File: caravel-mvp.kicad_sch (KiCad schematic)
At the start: 47 parts, among them J2 Conn_01x02, J3 Conn_02x04_Odd_Even, J4 Conn_01x06, J6 Conn_02x18_Odd_Even, J6 USB_C_Receptacle_USB2.0, J9 613012243121, SW3 B3U-1000P, U1 Caravel_QFN, U1 W25Q32JVSS, X1 10MHz

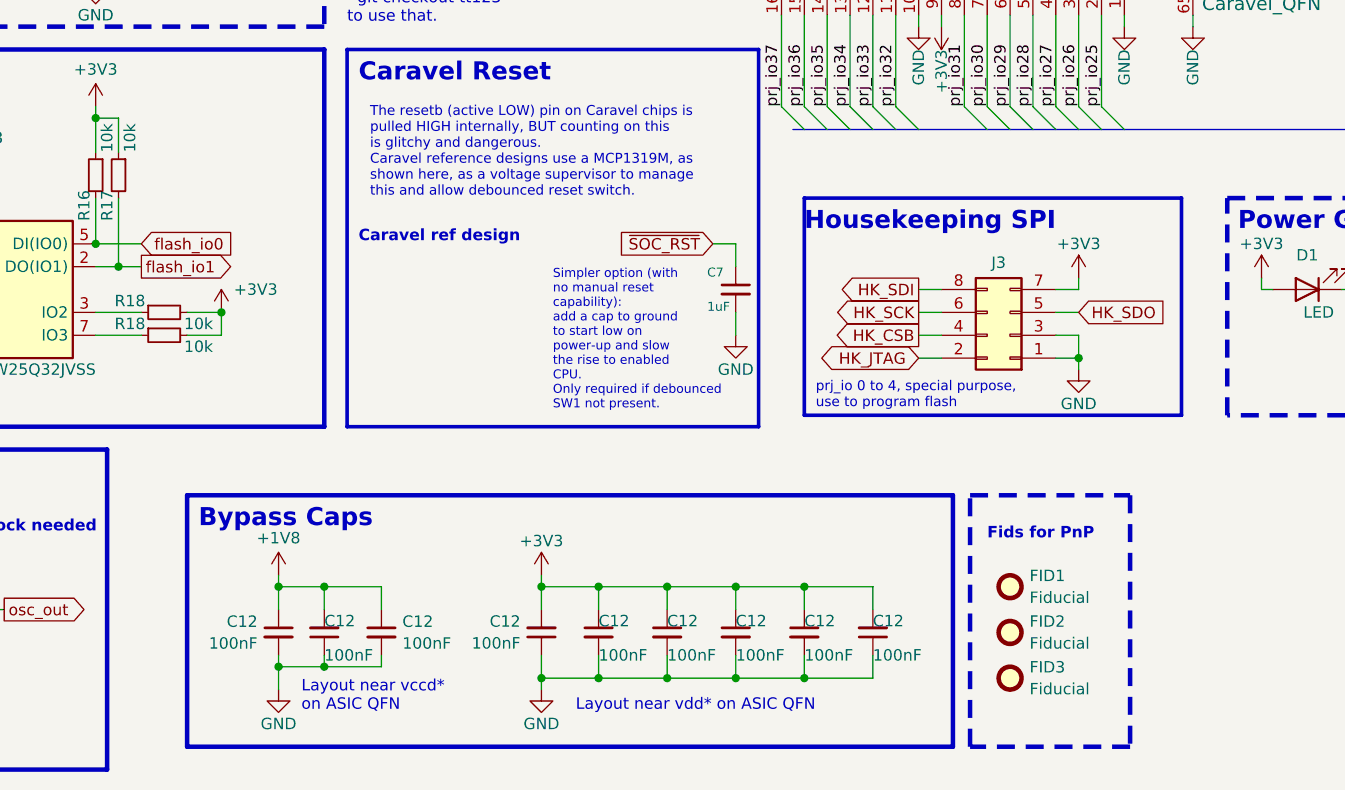
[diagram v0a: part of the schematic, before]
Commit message: Cleanups and even more clarifications in comments
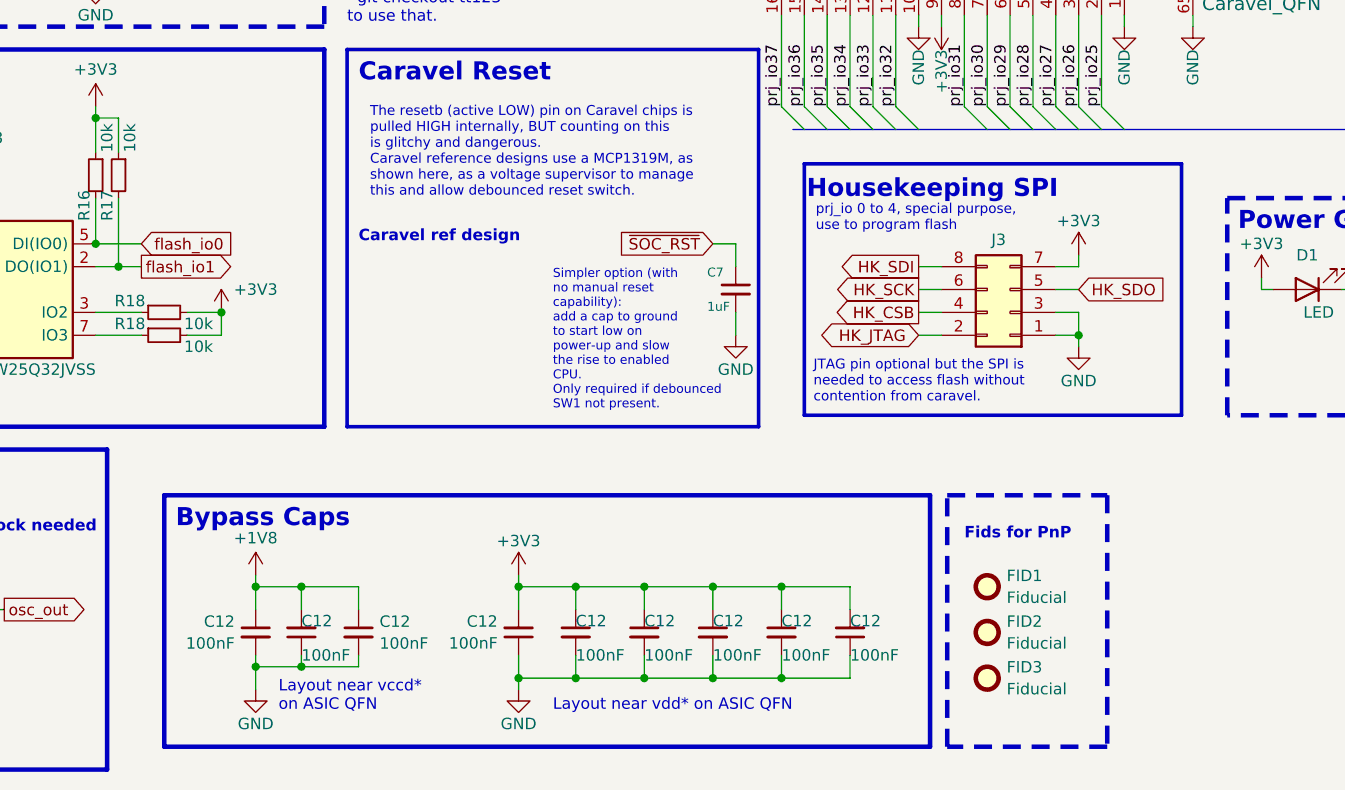
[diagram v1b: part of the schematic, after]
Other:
- note added: "JTAG pin optional but the SPI is needed to access flash without contention from caravel."
- moved on the sheet: C12, FID1, FID2, FID3, J3
